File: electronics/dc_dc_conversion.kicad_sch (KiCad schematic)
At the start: 18 parts, among them Q1 Q_NMOS_DGS, Q2 Q_PMOS_DGS, U1 TLV1117-33

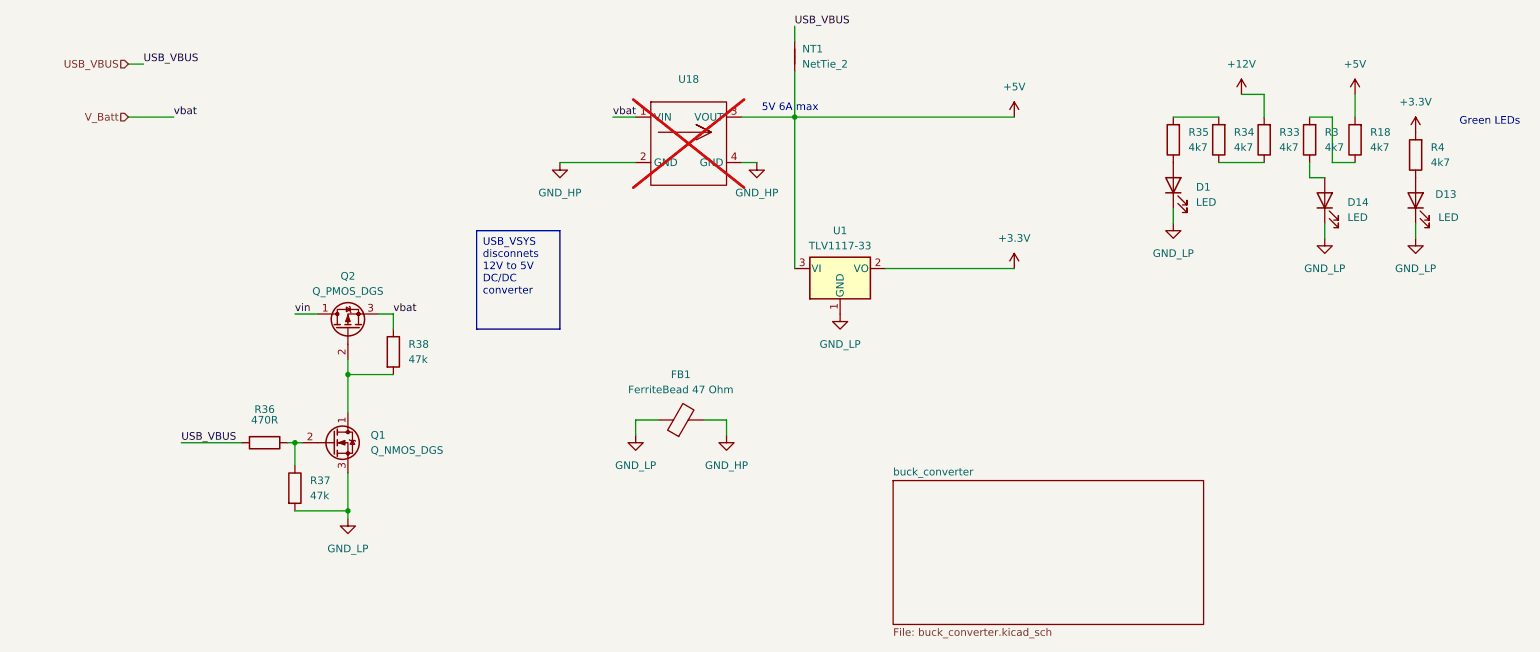
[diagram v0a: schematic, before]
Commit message: layouting progress. some 3d models upload
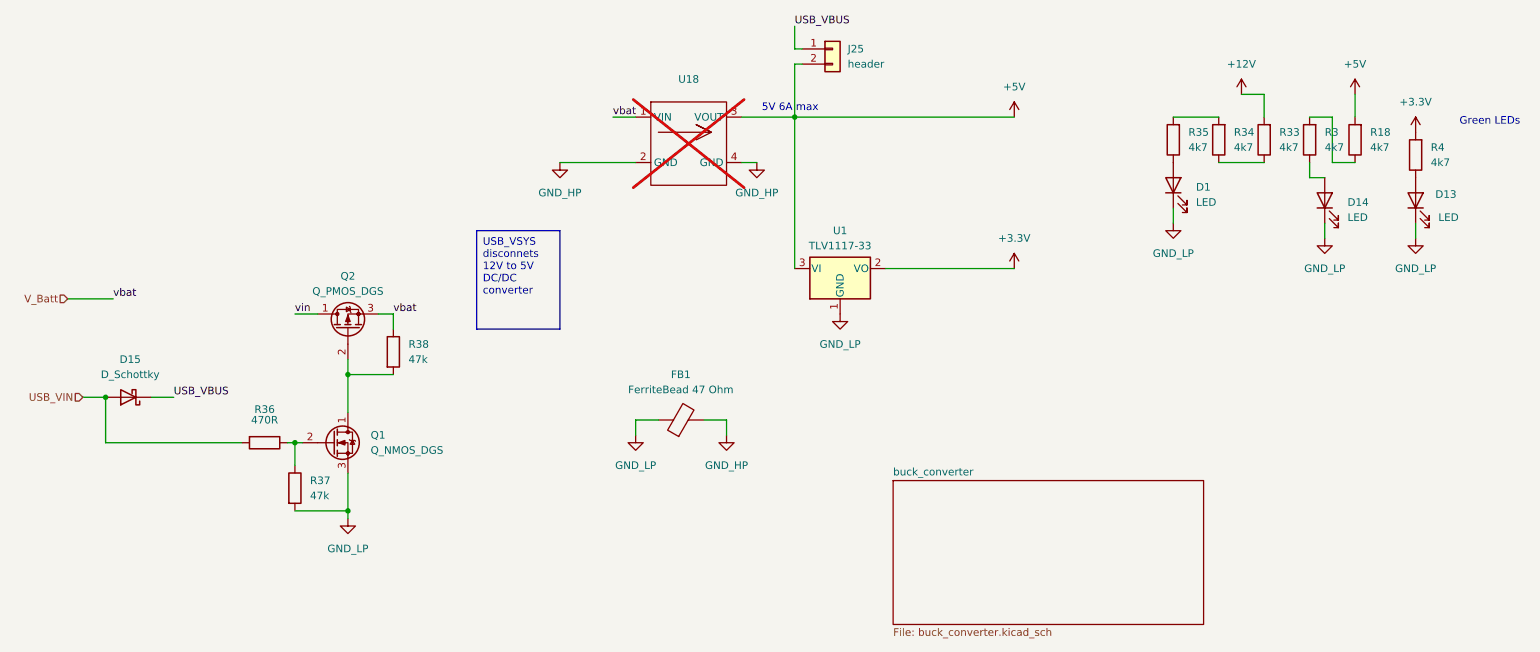
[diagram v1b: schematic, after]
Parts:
- removed NT1: NetTie_2, NetTie:NetTie-2_THT_Pad1.0mm, symbol Device:NetTie_2
- added D15: D_Schottky, Diode_SMD:D_SMA, symbol Device:D_Schottky
- added J25: header, Connector_PinHeader_2.54mm:PinHeader_1x02_P2.54mm_Vertical, symbol Connector_Generic:Conn_01x02
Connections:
- net +5V: now also J25.2 (Pin_2)
- net USB_VBUS: now also D15.1 (K), J25.1 (Pin_1); no longer R36.2
- new net USB_VIN: D15.2 (A), R36.2
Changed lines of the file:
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@@
 	(paper "A4")
+	(junction
+		(at 38.1 85.09)
+		(diameter 0)
+		(color 0 0 0 0)
+	)
 	(junction
 		(at 69.85 92.71)
@@
 	(wire
 		(pts
+			(xy 38.1 92.71) (xy 38.1 85.09)
+		)
+		(stroke
+			(width 0)
+			(type default)
+		)
+	)
+	(wire
+		(pts
 			(xy 242.57 55.88) (xy 242.57 58.42)
 		)
@@
 	(wire
 		(pts
+			(xy 154.94 26.67) (xy 153.67 26.67)
+		)
+		(stroke
+			(width 0)
+			(type default)
+		)
+	)
+	(wire
+		(pts
 			(xy 78.74 81.28) (xy 78.74 87.63)
 		)
@@
 	(wire
 		(pts
-			(xy 41.91 29.21) (xy 44.45 29.21)
+			(xy 34.29 85.09) (xy 38.1 85.09)
 		)
 		(stroke
@@
 	(wire
 		(pts
+			(xy 153.67 29.21) (xy 154.94 29.21)
+		)
+		(stroke
+			(width 0)
+			(type default)
+		)
+	)
+	(wire
+		(pts
 			(xy 68.58 92.71) (xy 69.85 92.71)
 		)
@@
 	(wire
 		(pts
-			(xy 41.91 38.1) (xy 49.53 38.1)
+			(xy 31.75 68.58) (xy 39.37 68.58)
 		)
 		(stroke
@@
 	(wire
 		(pts
-			(xy 153.67 22.86) (xy 153.67 25.4)
+			(xy 153.67 22.86) (xy 153.67 26.67)
 		)
 		(stroke
@@
 	(wire
 		(pts
+			(xy 45.72 85.09) (xy 49.53 85.09)
+		)
+		(stroke
+			(width 0)
+			(type default)
+		)
+	)
+	(wire
+		(pts
+			(xy 38.1 92.71) (xy 60.96 92.71)
+		)
+		(stroke
+			(width 0)
+			(type default)
+		)
+	)
+	(wire
+		(pts
 			(xy 142.24 88.9) (xy 138.43 88.9)
 		)
@@
 	(wire
 		(pts
+			(xy 153.67 29.21) (xy 153.67 38.1)
+		)
+		(stroke
+			(width 0)
+			(type default)
+		)
+	)
+	(wire
+		(pts
 			(xy 69.85 92.71) (xy 69.85 96.52)
 		)
@@
 	(wire
 		(pts
-			(xy 50.8 92.71) (xy 60.96 92.71)
-		)
-		(stroke
-			(width 0)
-			(type default)
-		)
-	)
-	(wire
-		(pts
 			(xy 114.3 45.72) (xy 127 45.72)
 		)
@@
 		(pts
 			(xy 123.19 38.1) (xy 127 38.1)
-		)
-		(stroke
-			(width 0)
-			(type default)
-		)
-	)
-	(wire
-		(pts
-			(xy 153.67 30.48) (xy 153.67 38.1)
 		)
 		(stroke
@@
 	)
 	(label "vbat"
-		(at 49.53 38.1 0)
+		(at 39.37 68.58 0)
+		(fields_autoplaced yes)
 		(effects
 			(font
@@
 	(label "vin"
 		(at 69.85 71.12 0)
+		(fields_autoplaced yes)
 		(effects
 			(font
@@
 		)
 	)
-	(label "vbat"
-		(at 86.36 71.12 0)
+	(label "USB_VBUS"
+		(at 49.53 85.09 0)
+		(fields_autoplaced yes)
 		(effects
 			(font
@@
 		)
 	)
-	(label "USB_VBUS"
-		(at 44.45 29.21 0)
+	(label "vbat"
+		(at 86.36 71.12 0)
+		(fields_autoplaced yes)
 		(effects
 			(font
@@
 	(label "USB_VBUS"
 		(at 153.67 22.86 0)
+		(fields_autoplaced yes)
 		(effects
 			(font
@@
 	(label "vbat"
 		(at 123.19 38.1 0)
+		(fields_autoplaced yes)
 		(effects
 			(font
@@
 		)
 	)
-	(label "USB_VBUS"
-		(at 50.8 92.71 0)
+	(hierarchical_label "V_Batt"
+		(shape input)
+		(at 31.75 68.58 180)
+		(fields_autoplaced yes)
 		(effects
 			(font
 				(size 1.27 1.27)
 			)
-			(justify left bottom)
-		)
-	)
-	(hierarchical_label "V_Batt"
+			(justify right)
+		)
+	)
+	(hierarchical_label "USB_VIN"
 		(shape input)
-		(at 41.91 38.1 180)
+		(at 34.29 85.09 180)
+		(fields_autoplaced yes)
 		(effects
 			(font
@@
 		)
 	)
-	(hierarchical_label "USB_VBUS"
-		(shape input)
-		(at 41.91 29.21 180)
-		(effects
-			(font
-				(size 1.27 1.27)
-			)
-			(justify right)
-		)
-	)
 	(symbol
 		(lib_id "Device:R")
@@
 	)
 	(symbol
+		(lib_id "Connector_Generic:Conn_01x02")
+		(at 160.02 26.67 0)
+		(unit 1)
+		(exclude_from_sim no)
+		(in_bom yes)
+		(on_board yes)
+		(dnp no)
+		(fields_autoplaced yes)
+		(property "Reference" "J25"
+			(at 162.56 26.6699 0)
+			(effects
+				(font
+					(size 1.27 1.27)
+				)
+				(justify left)
+			)
+		)
+		(property "Value" "header"
+			(at 162.56 29.2099 0)
+			(effects
+				(font
+					(size 1.27 1.27)
+				)
+				(justify left)
+			)
+		)
+		(property "Footprint" "Connector_PinHeader_2.54mm:PinHeader_1x02_P2.54mm_Vertical"
+			(at 160.02 26.67 0)
+			(effects
+				(font
+					(size 1.27 1.27)
+				)
+				(hide yes)
+			)
+		)
+		(property "Datasheet" "~"
+			(at 160.02 26.67 0)
+			(effects
+				(font
+					(size 1.27 1.27)
+				)
+				(hide yes)
+			)
+		)
+		(property "Description" "Generic connector, single row, 01x02, script generated (kicad-library-utils/schlib/autogen/connector/)"
+			(at 160.02 26.67 0)
+			(effects
+				(font
+					(size 1.27 1.27)
+				)
+				(hide yes)
+			)
+		)
+		(pin "1"
+		)
+		(pin "2"
+		)
+		(instances
+			(project ""
+				(path "/eeb1234c-eae0-4ac6-a30d-2a978d66d889/04c402f1-b99a-4823-99a0-0c7312782f29/e988bf0b-0303-4560-abbf-9db3a1d13611"
+					(reference "J25")
+					(unit 1)
+				)
+			)
+		)
+	)
+	(symbol
 		(lib_id "power:GND2")
 		(at 217.17 55.88 0)
@@
 	)
 	(symbol
-		(lib_id "Device:NetTie_2")
-		(at 153.67 27.94 90)
-		(unit 1)
-		(exclude_from_sim no)
-		(in_bom no)
-		(on_board yes)
-		(dnp no)
-		(fields_autoplaced yes)
-		(property "Reference" "NT1"
-			(at 154.94 26.6699 90)
-			(effects
-				(font
-					(size 1.27 1.27)
-				)
-				(justify right)
-			)
-		)
-		(property "Value" "NetTie_2"
-			(at 154.94 29.2099 90)
-			(effects
-				(font
-					(size 1.27 1.27)
-				)
-				(justify right)
-			)
-		)
-		(property "Footprint" "NetTie:NetTie-2_THT_Pad1.0mm"
-			(at 153.67 27.94 0)
-			(effects
-				(font
-					(size 1.27 1.27)
-				)
-				(hide yes)
-			)
-		)
-		(property "Datasheet" "~"
-			(at 153.67 27.94 0)
-			(effects
-				(font
-					(size 1.27 1.27)
-				)
-				(hide yes)
-			)
-		)
-		(property "Description" "Net tie, 2 pins"
-			(at 153.67 27.94 0)
-			(effects
-				(font
-					(size 1.27 1.27)
-				)
-				(hide yes)
-			)
-		)
-		(pin "2"
-		)
-		(pin "1"
-		)
-		(instances
-			(project "electronics"
-				(path "/eeb1234c-eae0-4ac6-a30d-2a978d66d889/04c402f1-b99a-4823-99a0-0c7312782f29/e988bf0b-0303-4560-abbf-9db3a1d13611"
-					(reference "NT1")
-					(unit 1)
-				)
-			)
-		)
-	)
-	(symbol
 		(lib_id "Device:R")
 		(at 86.36 77.47 0)
@@
 					(unit 1)
 				)
+			)
+		)
+	)
+	(symbol
+		(lib_id "Device:D_Schottky")
+		(at 41.91 85.09 180)
+		(unit 1)
+		(exclude_from_sim no)
+		(in_bom yes)
+		(on_board yes)
+		(dnp no)
+		(fields_autoplaced yes)
+		(property "Reference" "D15"
+			(at 42.2275 78.74 0)
+			(effects
+				(font
+					(size 1.27 1.27)
+				)
+			)
+		)
+		(property "Value" "D_Schottky"
+			(at 42.2275 81.28 0)
+			(effects
+				(font
+					(size 1.27 1.27)
+				)
+			)
+		)
+		(property "Footprint" "Diode_SMD:D_SMA"
+			(at 41.91 85.09 0)
+			(effects
+				(font
+					(size 1.27 1.27)
+				)
+				(hide yes)
+			)
+		)
+		(property "Datasheet" "~"
+			(at 41.91 85.09 0)
+			(effects
+				(font
+					(size 1.27 1.27)
+				)
+				(hide yes)
+			)
+		)
+		(property "Description" "Schottky diode"
+			(at 41.91 85.09 0)
+			(effects
+				(font
+					(size 1.27 1.27)
+				)
+				(hide yes)
+			)
+		)
+		(pin "1"
+		)
+		(pin "2"
+		)
+		(instances
+			(project "electronics"
+				(path "/eeb1234c-eae0-4ac6-a30d-2a978d66d889/04c402f1-b99a-4823-99a0-0c7312782f29/e988bf0b-0303-4560-abbf-9db3a1d13611"
+					(reference "D15")
+					(unit 1)
+				)
